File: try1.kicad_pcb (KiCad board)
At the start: 2 copper layers, 175.3 x 119.4 mm, 33 parts, among them J10 Archon-connector-modules-Driv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, J11 Archon-connector-modules-Driv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, J2 Archon-connector-modules-Heat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, J21 DB37, J22 DB37, J3 Archon-connector-modules-Driv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, J31 DB9, J4 Archon-connector-modules-LVBi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, J41 CONN_DVI, J5 Archon-connector-modules-ADC, J6 Archon-connector-modules-ADC, J7 Archon-connector-modules-ADC, J8 Archon-connector-modules-ADC, J9 Archon-connector-modules-HVBi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, P1 CONN_02X02

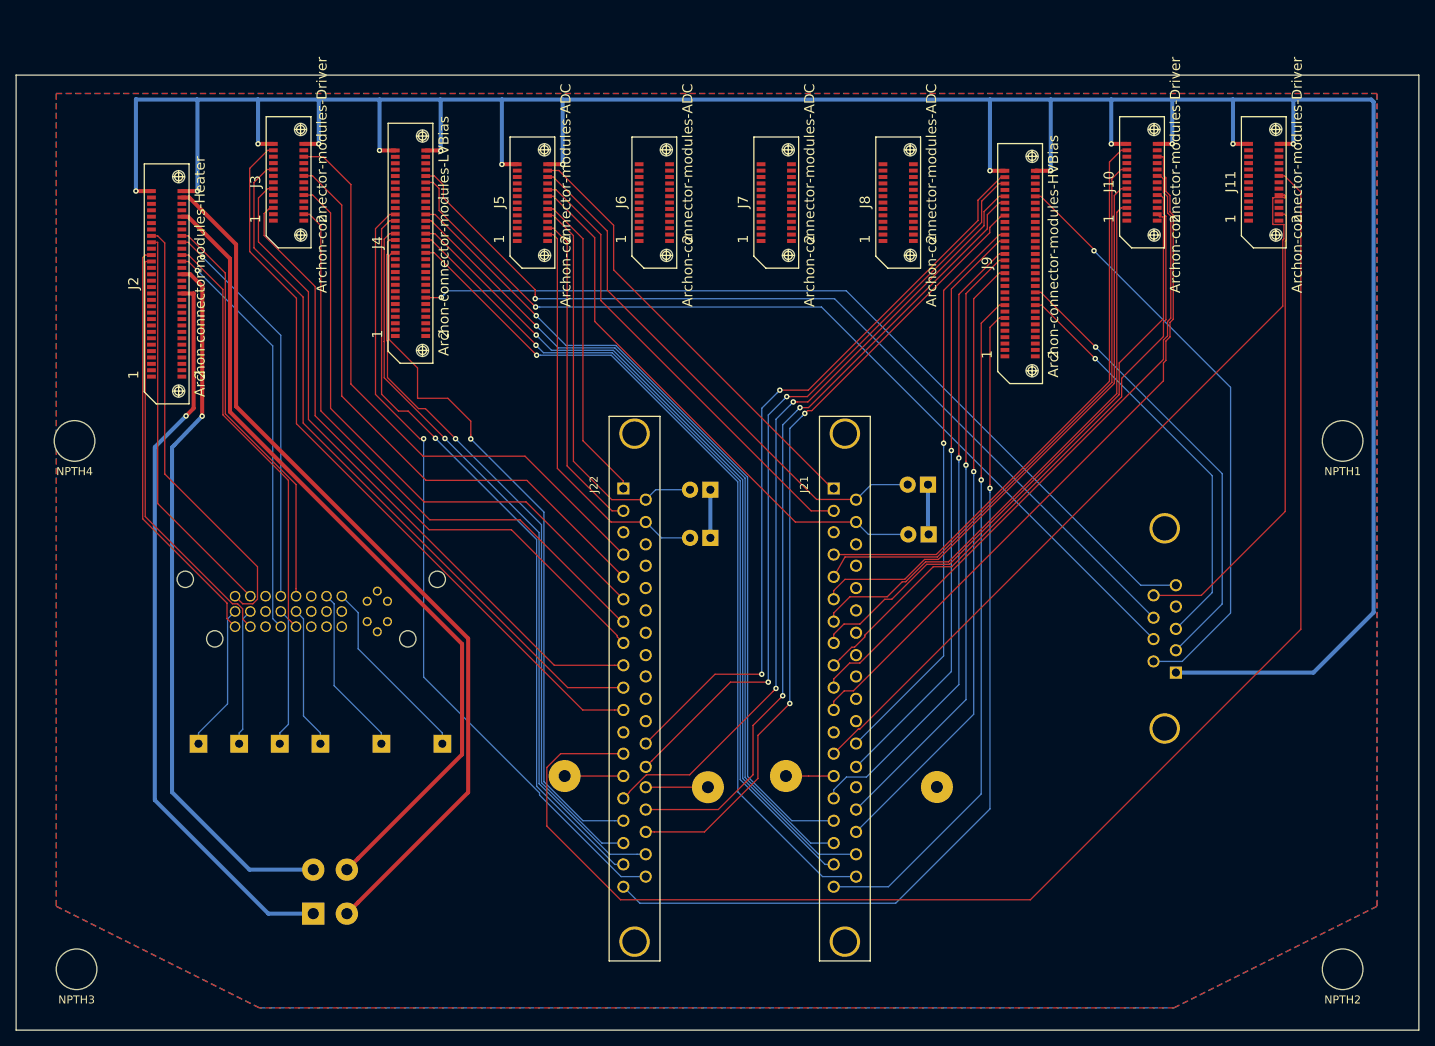
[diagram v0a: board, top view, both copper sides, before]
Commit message: PCB Layout Fix-Ups
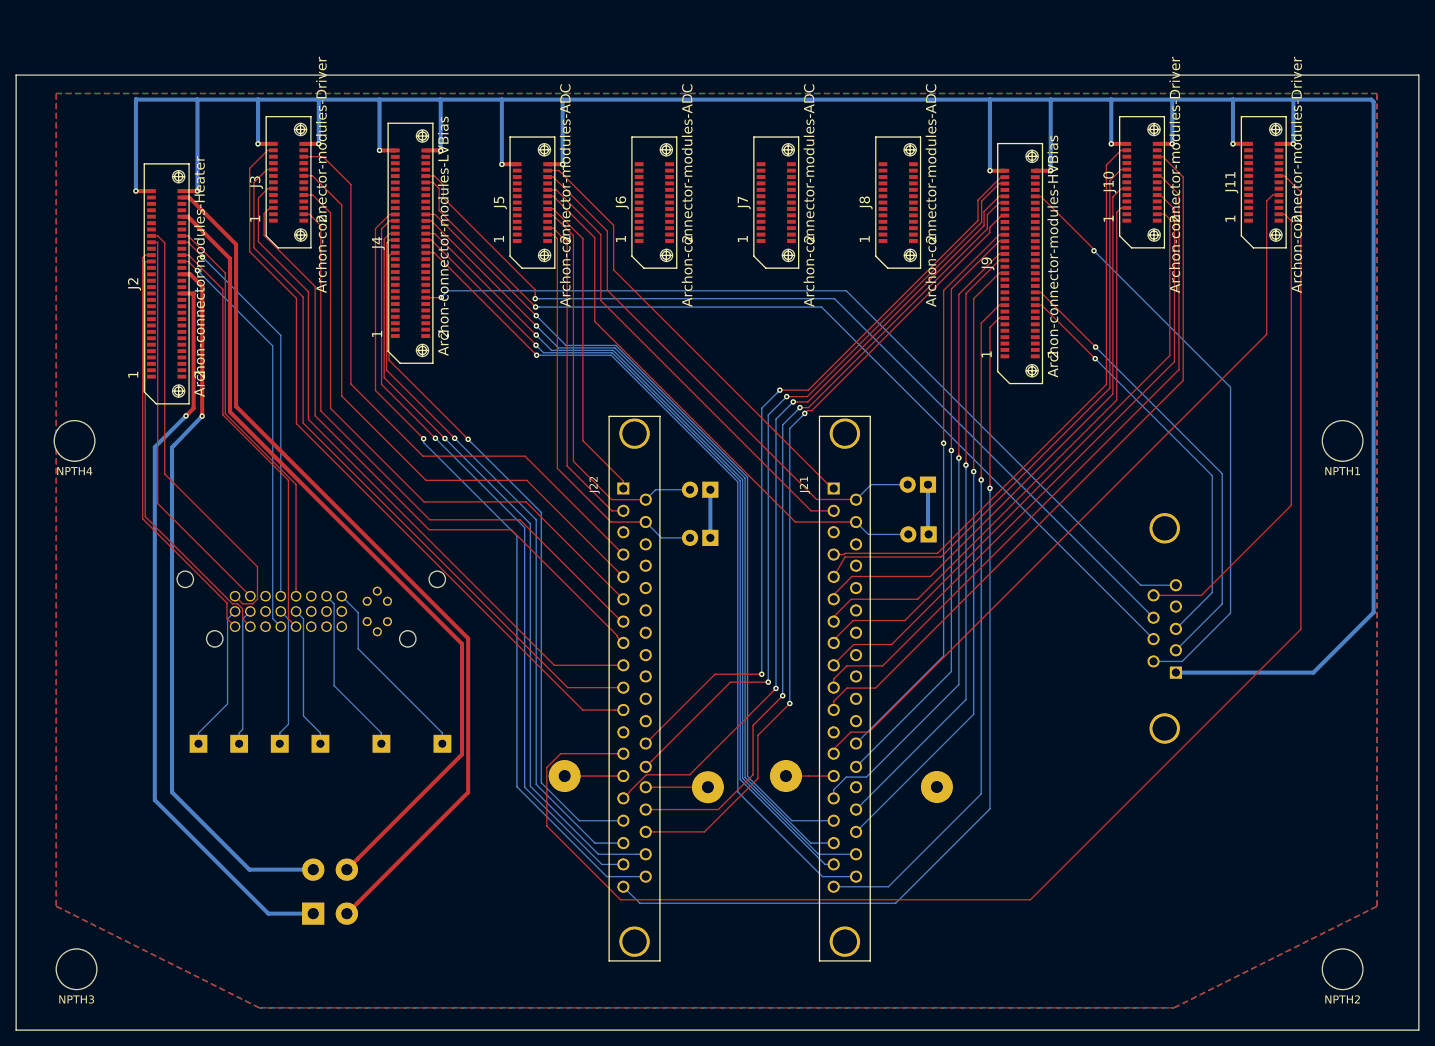
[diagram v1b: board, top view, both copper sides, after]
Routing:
- net /~ResetLog_R: track 97.7 -> 94.7 mm
- net /P3X: track 83.1 -> 85.8 mm
- net /TGX: track 88.7 -> 91.1 mm
- net /P2X: track 78.2 -> 80.3 mm
- net /VLg_L: track 88.9 -> 86.9 mm
- net /P1X: track 74.6 -> 76.0 mm
- net /ResetLO_L: track 94.7 -> 95.6 mm
- net /-15V_L: track 100.3 -> 101.1 mm
- net FLASH_V: track 58.8 -> 59.3 mm
